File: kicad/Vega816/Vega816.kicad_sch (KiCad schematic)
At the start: 4 parts

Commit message: Big push, Sysctl, DMA Reg
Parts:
- removed U? (x4): BB816Breakout, symbol Vega816:BB816Breakout
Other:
- removed sheet CPU Buffer0
- removed sheet CPU Buffer1
- removed sheet CPU Buffer10
- removed sheet CPU Buffer11
- removed sheet CPU Buffer12
- removed sheet CPU Buffer13
- removed sheet CPU Buffer14
- removed sheet CPU Buffer15
- removed sheet CPU Buffer2
- removed sheet CPU Buffer3
- removed sheet CPU Buffer4
- removed sheet CPU Buffer5
- removed sheet CPU Buffer6
- removed sheet CPU Buffer7
- removed sheet CPU Buffer8
- removed sheet CPU Buffer9
- removed sheet CPU Shim A
- removed sheet CPU Shim B
- removed sheet CPU Shim C
- removed sheet CPU Shim D
- removed sheet DMA Controller
- removed sheet Device Port
- note removed: "32KB EEPROM"
- note removed: "DMA 0"
- note removed: "DMA 1"
- note removed: "DMA 2"
- note removed: "DMA 3"
- note removed: "DMA Channels"
- note removed: "Four CPUs x 4 DMA Channels"
- note removed: "Vega 816 SMP Computer System"

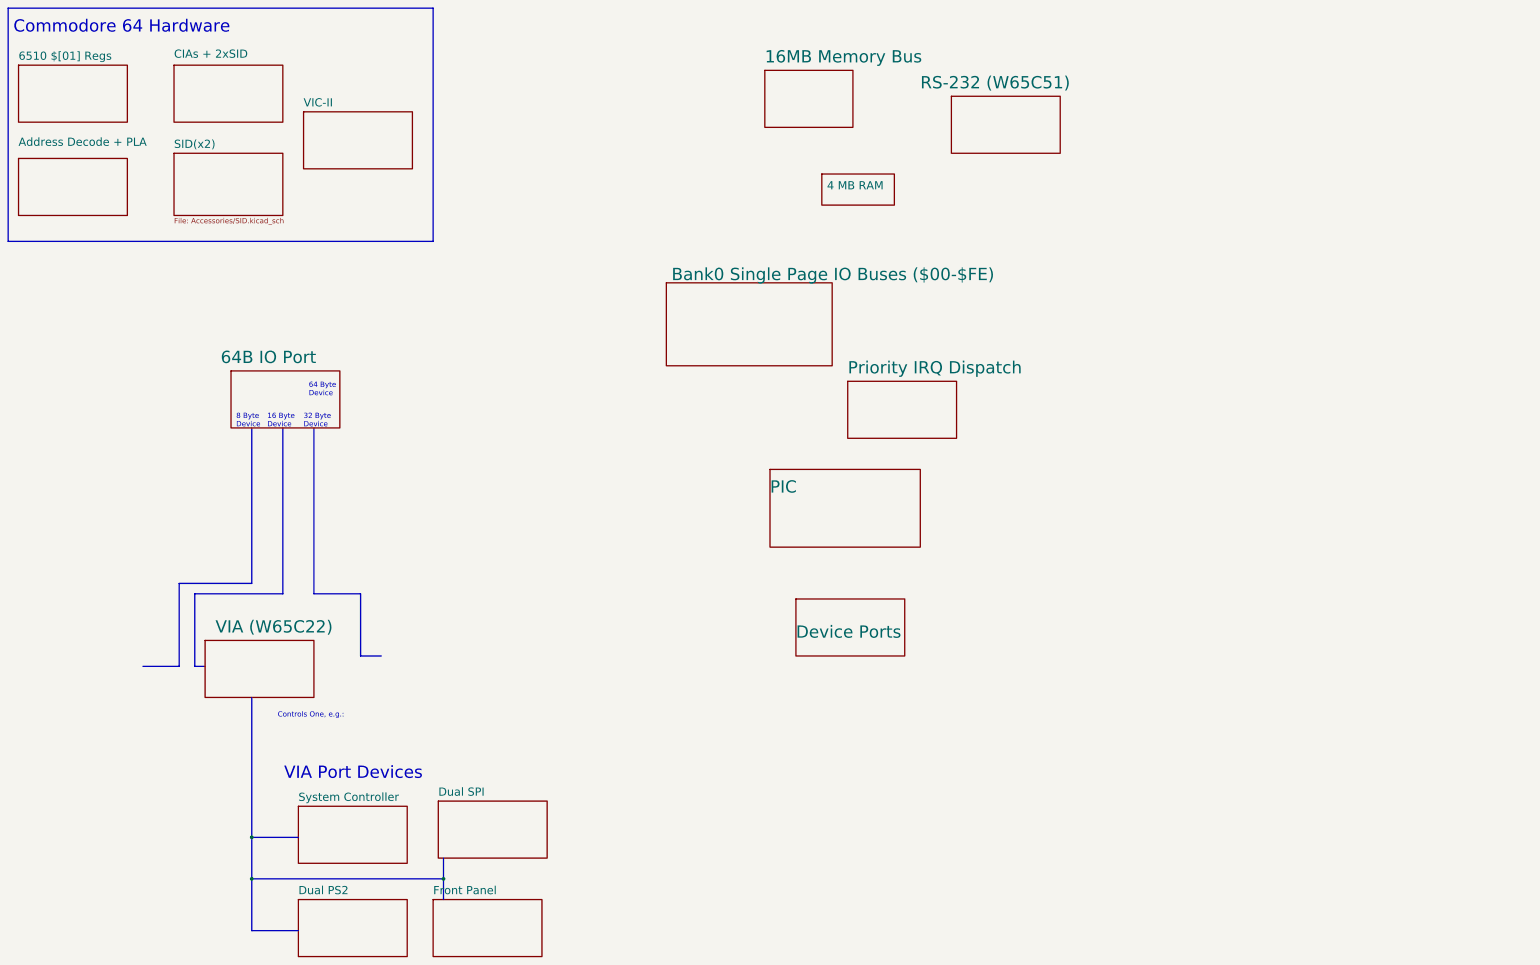
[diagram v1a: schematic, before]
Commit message: Big
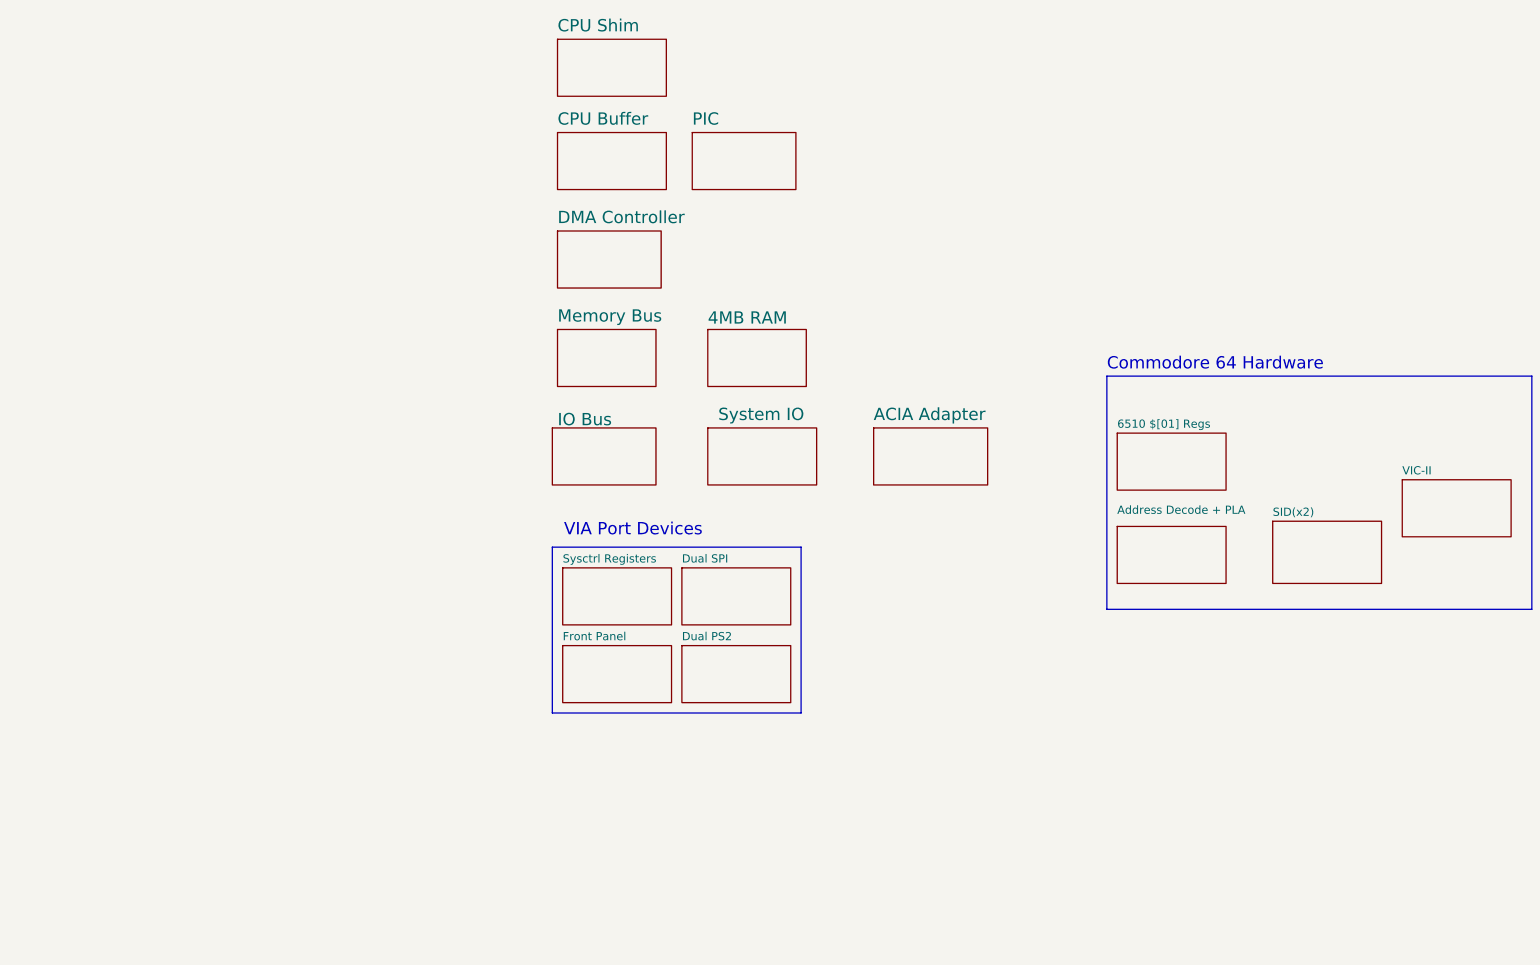
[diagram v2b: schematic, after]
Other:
- sheet 16MB Memory Bus renamed Memory Bus
- sheet 4 MB RAM renamed 4MB RAM
- sheet Bank0 Single Page IO Buses ($00-$FE) renamed IO Bus
- sheet System Controller renamed Sysctrl Registers
- sheet VIA (W65C22) renamed System IO
- removed sheet 64B IO Port
- removed sheet CIAs + 2xSID
- removed sheet Device Ports
- removed sheet Priority IRQ Dispatch
- removed sheet RS-232 (W65C51)
- added sheet ACIA Adapter (Accessories/ACIAAdapter.kicad_sch)
- added sheet CPU Buffer (CPU Buffer/CPU Buffer.kicad_sch)
- added sheet CPU Shim (CPUShim/CPUShim.kicad_sch)
- added sheet DMA Controller (DMAController/DMAController.kicad_sch)
- sheet IO Bus: file MemoryExpansionBus/irq_multiplex.kicad_sch -> IOBus/IOBus.kicad_sch
- note removed: "16 Byte Device"
- note removed: "32 Byte Device"
- note removed: "64 Byte Device"
- note removed: "8 Byte Device"
- note removed: "Controls One, e.g.:"
